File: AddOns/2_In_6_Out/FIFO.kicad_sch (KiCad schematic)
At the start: 10 parts, among them U2 5PB1213NTGK8, U4 5PB1213NTGK8

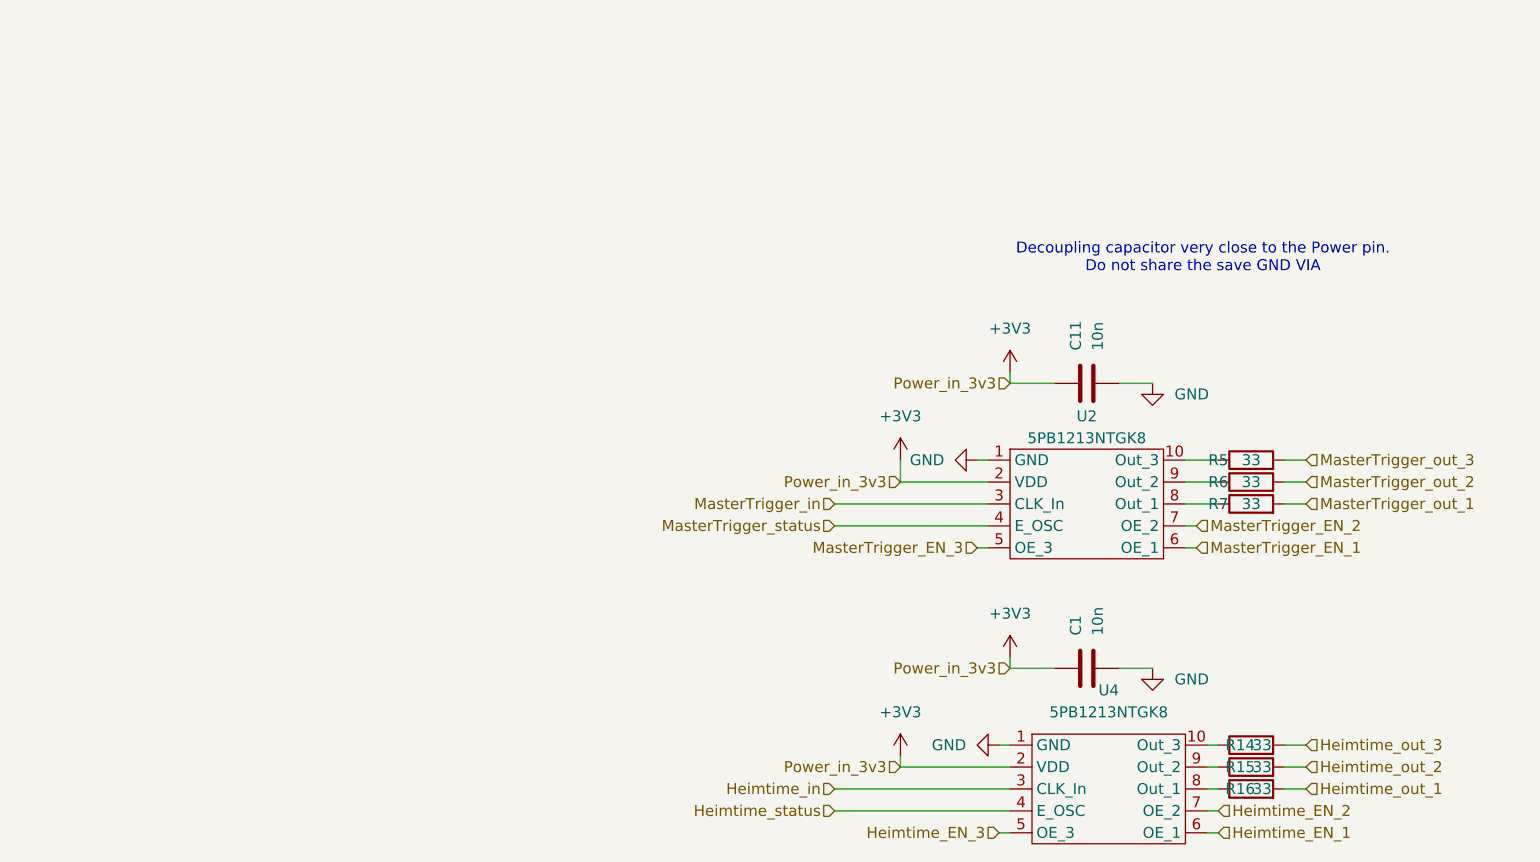
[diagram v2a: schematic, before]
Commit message: .
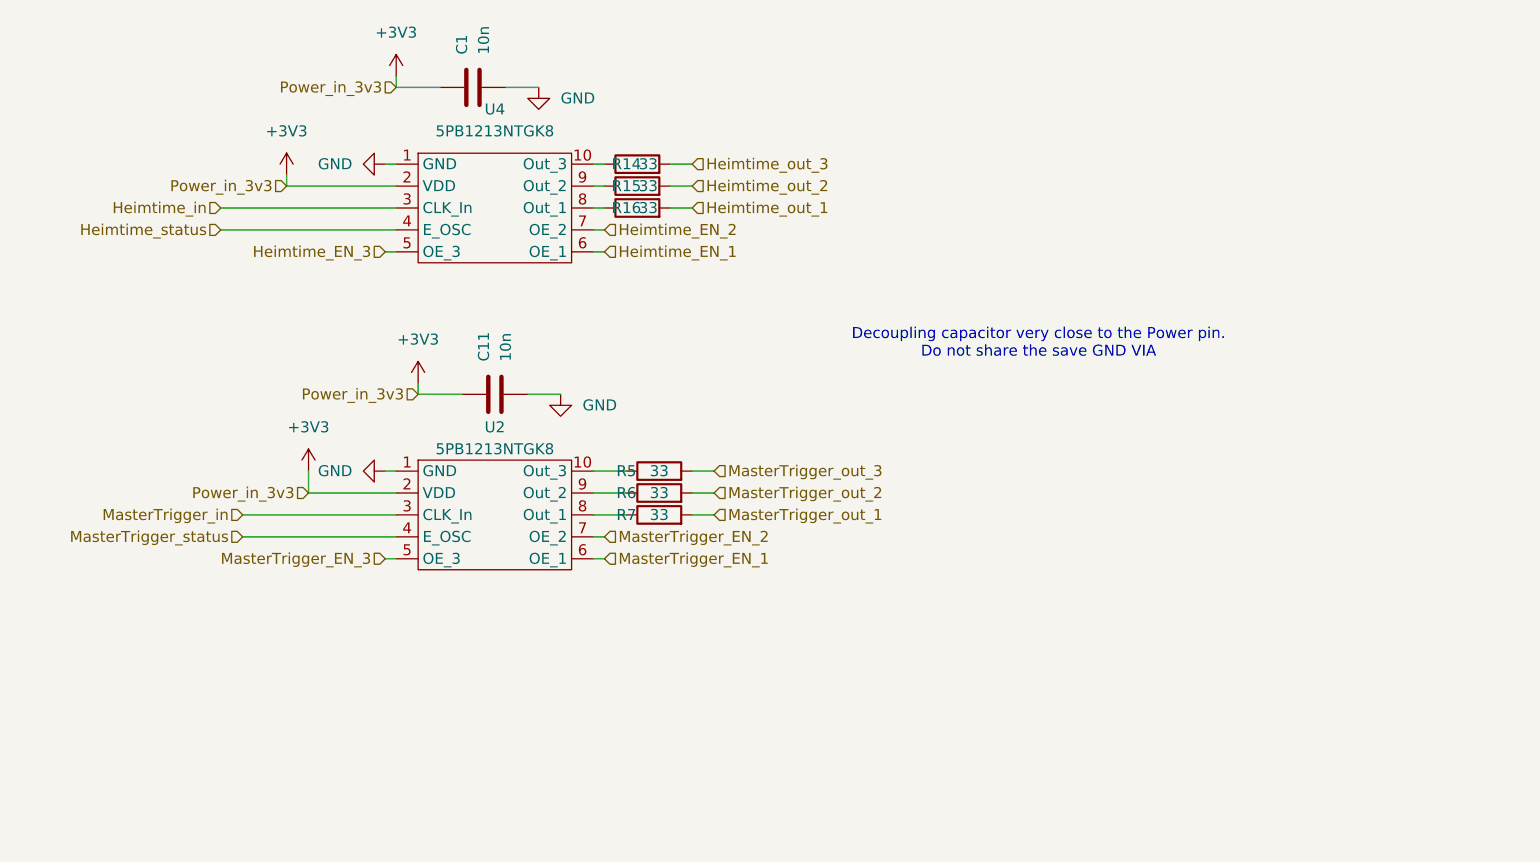
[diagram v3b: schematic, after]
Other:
- moved on the sheet: C1, C11, R14, R15, R16, R5, R6, R7, U2, U4
